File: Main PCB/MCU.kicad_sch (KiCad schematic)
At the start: 36 parts, among them J10 Conn_01x04, J11 Conn_01x04, J4 Conn_01x04, J5 Conn_01x04, J6 Conn_01x04, J7 Conn_01x04, J8 Conn_01x04, J9 Conn_01x04, U2 AT32F423CxU7, U3 AT32F423CxU7, U4 AT32F423CxU7, U5 AT32F423CxU7

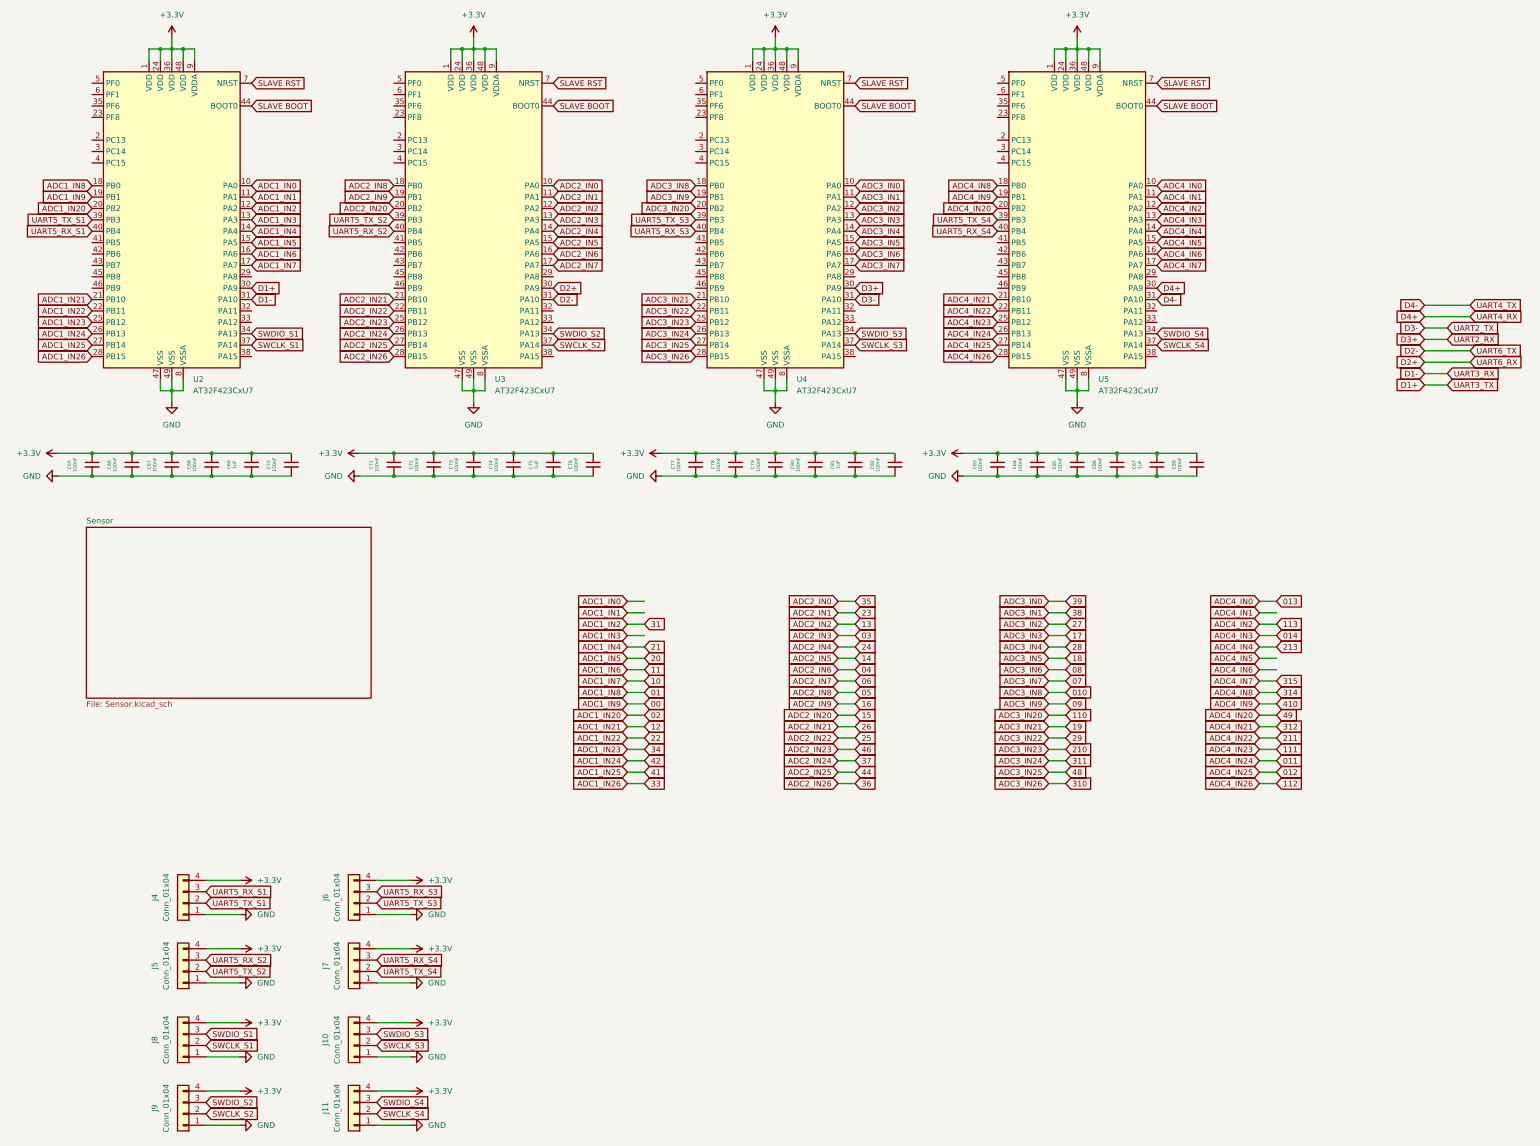
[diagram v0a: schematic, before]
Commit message: Revert "Initial Push"
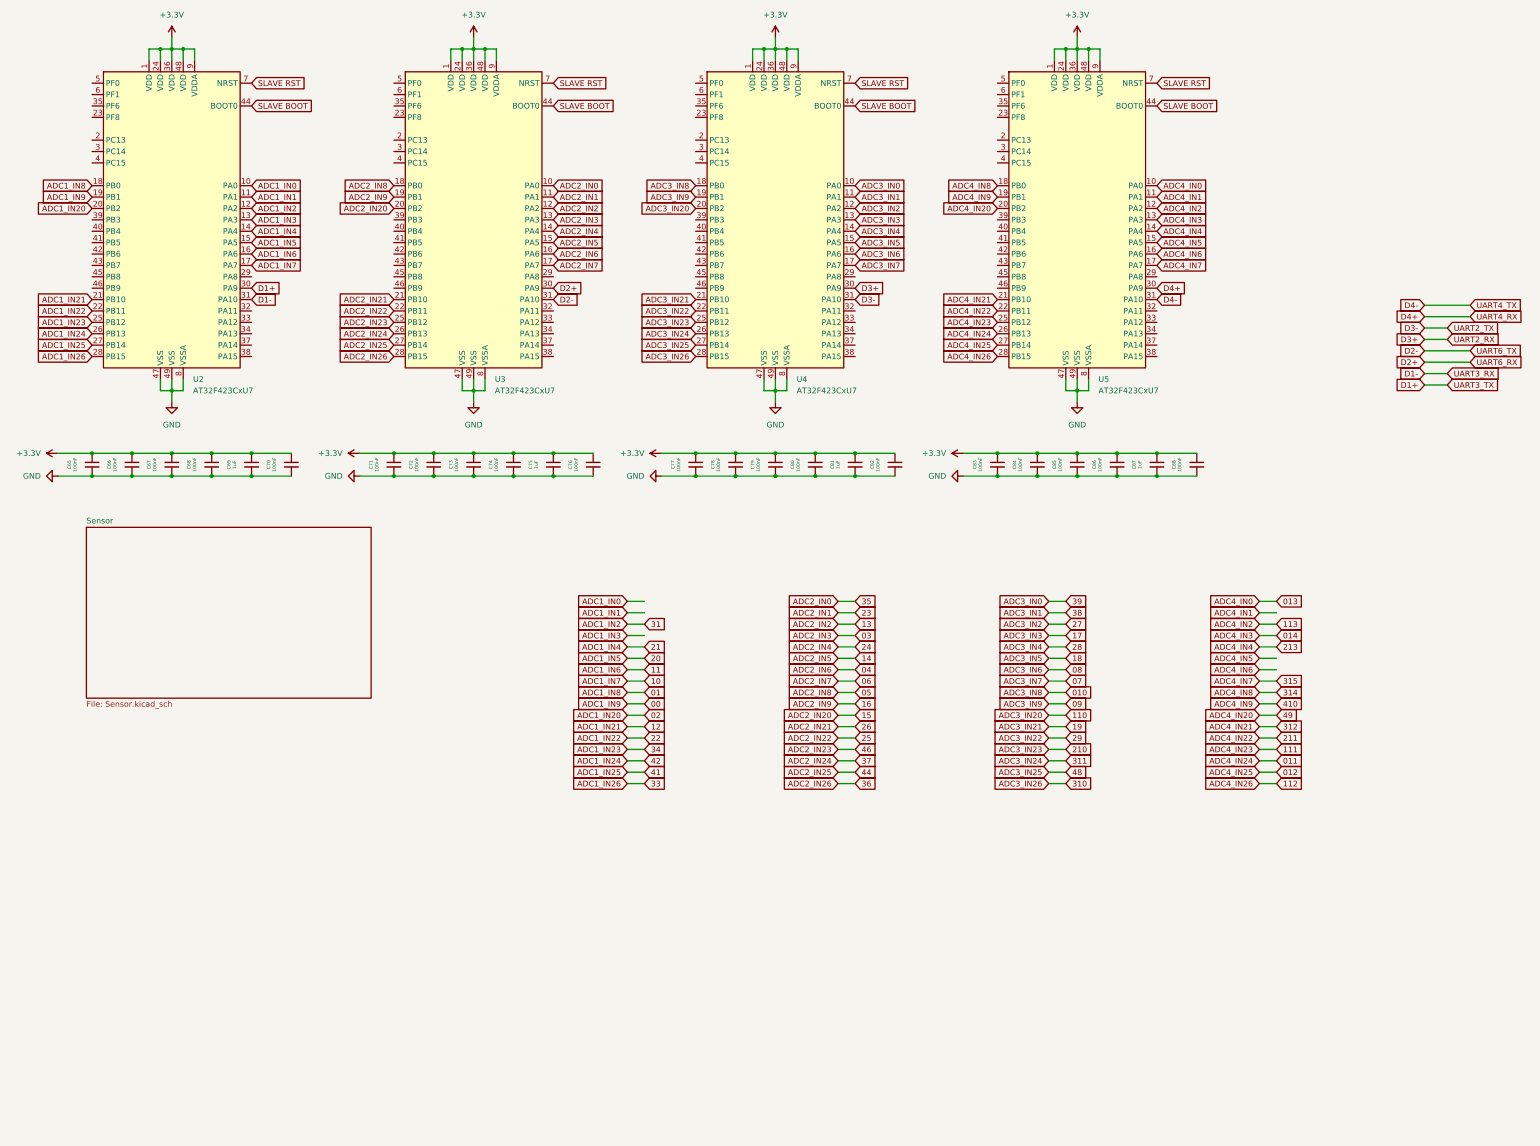
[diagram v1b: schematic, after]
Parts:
- removed J10, J11, J4, J5, J6, J7, J8, J9: Conn_01x04, Connector_PinHeader_2.54mm:PinHeader_1x04_P2.54mm_Vertical, symbol Connector_Generic:Conn_01x04
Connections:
- net SWCLK_S1: no longer names the net of U2.37 (PA14)
- net SWCLK_S2: no longer names the net of U3.37 (PA14)
- net SWCLK_S3: no longer names the net of U4.37 (PA14)
- net SWCLK_S4: no longer names the net of U5.37 (PA14)
- net SWDIO_S1: no longer names the net of U2.34 (PA13)
- net SWDIO_S2: no longer names the net of U3.34 (PA13)
- net SWDIO_S3: no longer names the net of U4.34 (PA13)
- net SWDIO_S4: no longer names the net of U5.34 (PA13)
- net UART5_RX_S1: no longer names the net of U2.40 (PB4)
- net UART5_RX_S2: no longer names the net of U3.40 (PB4)
- net UART5_RX_S3: no longer names the net of U4.40 (PB4)
- net UART5_RX_S4: no longer names the net of U5.40 (PB4)
- net UART5_TX_S1: no longer names the net of U2.39 (PB3)
- net UART5_TX_S2: no longer names the net of U3.39 (PB3)
- net UART5_TX_S3: no longer names the net of U4.39 (PB3)
- net UART5_TX_S4: no longer names the net of U5.39 (PB3)

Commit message: Initial Push
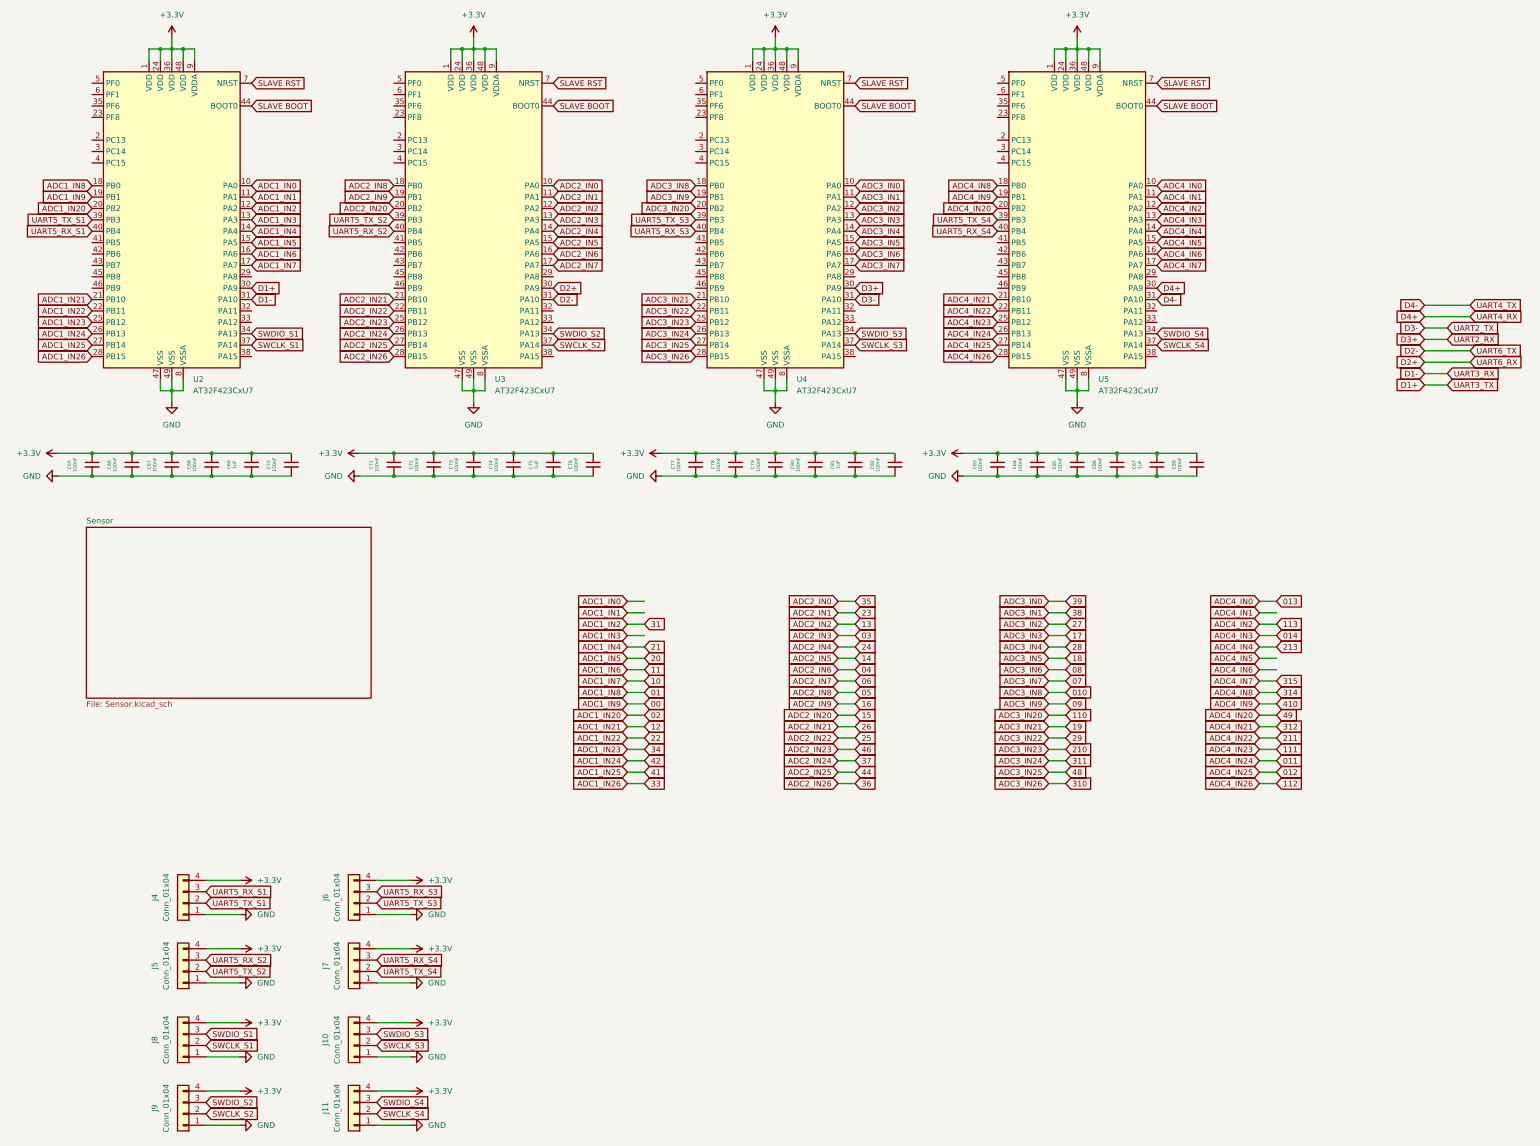
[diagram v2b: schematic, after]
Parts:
- added J10, J11, J4, J5, J6, J7, J8, J9: Conn_01x04, Connector_PinHeader_2.54mm:PinHeader_1x04_P2.54mm_Vertical, symbol Connector_Generic:Conn_01x04
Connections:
- net +3.3V: now also J10.4 (Pin_4), J11.4 (Pin_4), J4.4 (Pin_4), J5.4 (Pin_4), J6.4 (Pin_4), J7.4 (Pin_4), J8.4 (Pin_4), J9.4 (Pin_4)
- net GND: now also J10.1 (Pin_1), J11.1 (Pin_1), J4.1 (Pin_1), J5.1 (Pin_1), J6.1 (Pin_1), J7.1 (Pin_1), J8.1 (Pin_1), J9.1 (Pin_1)
- net SWDIO_S1: now reaches U2.34 (PA13)
- net SWDIO_S1: now also J8.3 (Pin_3)
- net SWCLK_S1: now reaches U2.37 (PA14)
- net SWCLK_S1: now also J8.2 (Pin_2)
- net UART5_TX_S1: now reaches U2.39 (PB3)
- net UART5_TX_S1: now also J4.2 (Pin_2)
- net UART5_RX_S1: now reaches U2.40 (PB4)
- net UART5_RX_S1: now also J4.3 (Pin_3)
- net SWDIO_S2: now reaches U3.34 (PA13)
- net SWDIO_S2: now also J9.3 (Pin_3)
- net SWCLK_S2: now reaches U3.37 (PA14)
- net SWCLK_S2: now also J9.2 (Pin_2)
- net UART5_TX_S2: now reaches U3.39 (PB3)
- net UART5_TX_S2: now also J5.2 (Pin_2)
- net UART5_RX_S2: now reaches U3.40 (PB4)
- net UART5_RX_S2: now also J5.3 (Pin_3)
- net SWDIO_S3: now reaches U4.34 (PA13)
- net SWDIO_S3: now also J10.3 (Pin_3)
- net SWCLK_S3: now reaches U4.37 (PA14)
- net SWCLK_S3: now also J10.2 (Pin_2)
- net UART5_TX_S3: now reaches U4.39 (PB3)
- net UART5_TX_S3: now also J6.2 (Pin_2)
- net UART5_RX_S3: now reaches U4.40 (PB4)
- net UART5_RX_S3: now also J6.3 (Pin_3)
- net SWDIO_S4: now reaches U5.34 (PA13)
- net SWDIO_S4: now also J11.3 (Pin_3)
- net SWCLK_S4: now reaches U5.37 (PA14)
- net SWCLK_S4: now also J11.2 (Pin_2)
- net UART5_TX_S4: now reaches U5.39 (PB3)
- net UART5_TX_S4: now also J7.2 (Pin_2)
- net UART5_RX_S4: now reaches U5.40 (PB4)
- net UART5_RX_S4: now also J7.3 (Pin_3)
